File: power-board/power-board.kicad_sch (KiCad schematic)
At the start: 23 parts, among them J1 LINE/LOAD, J2 DISPLAY, J3 PROG, K1 G3MB-202P, Q1 2N2222A, U1 HLK-PM01, U2 Arduino_pro_mini, U3 MAX6675

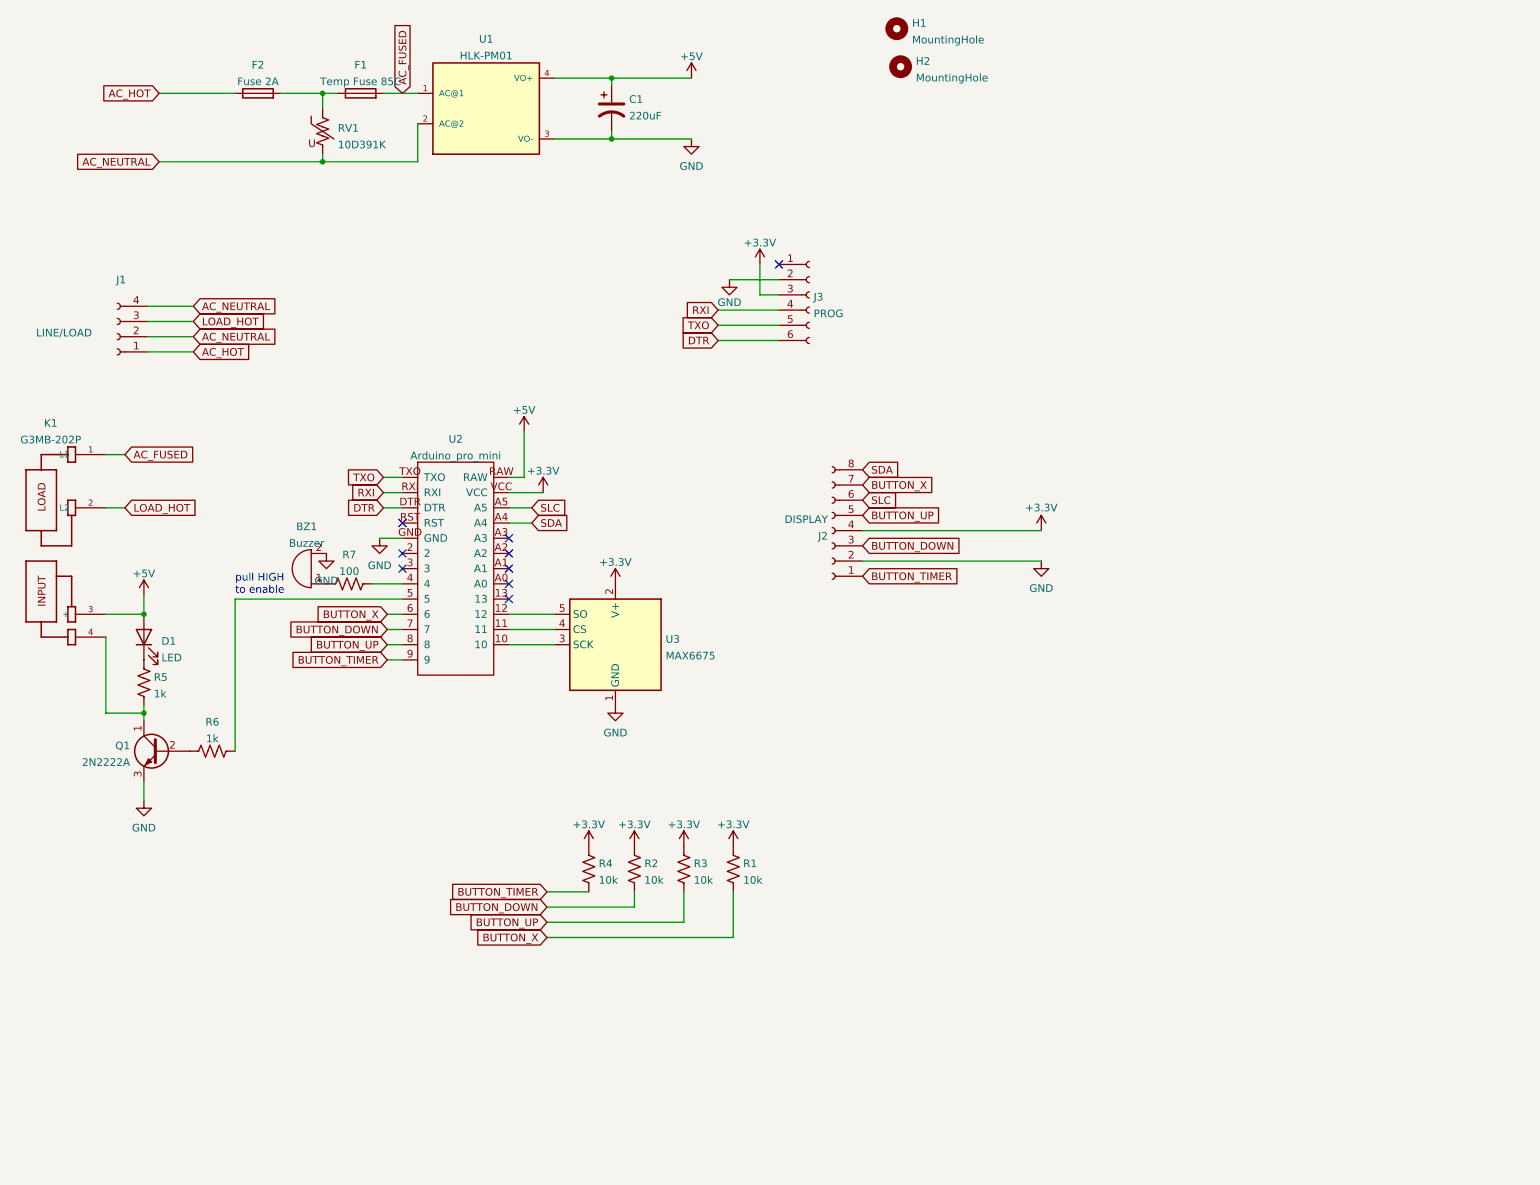
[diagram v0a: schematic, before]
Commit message: documentation
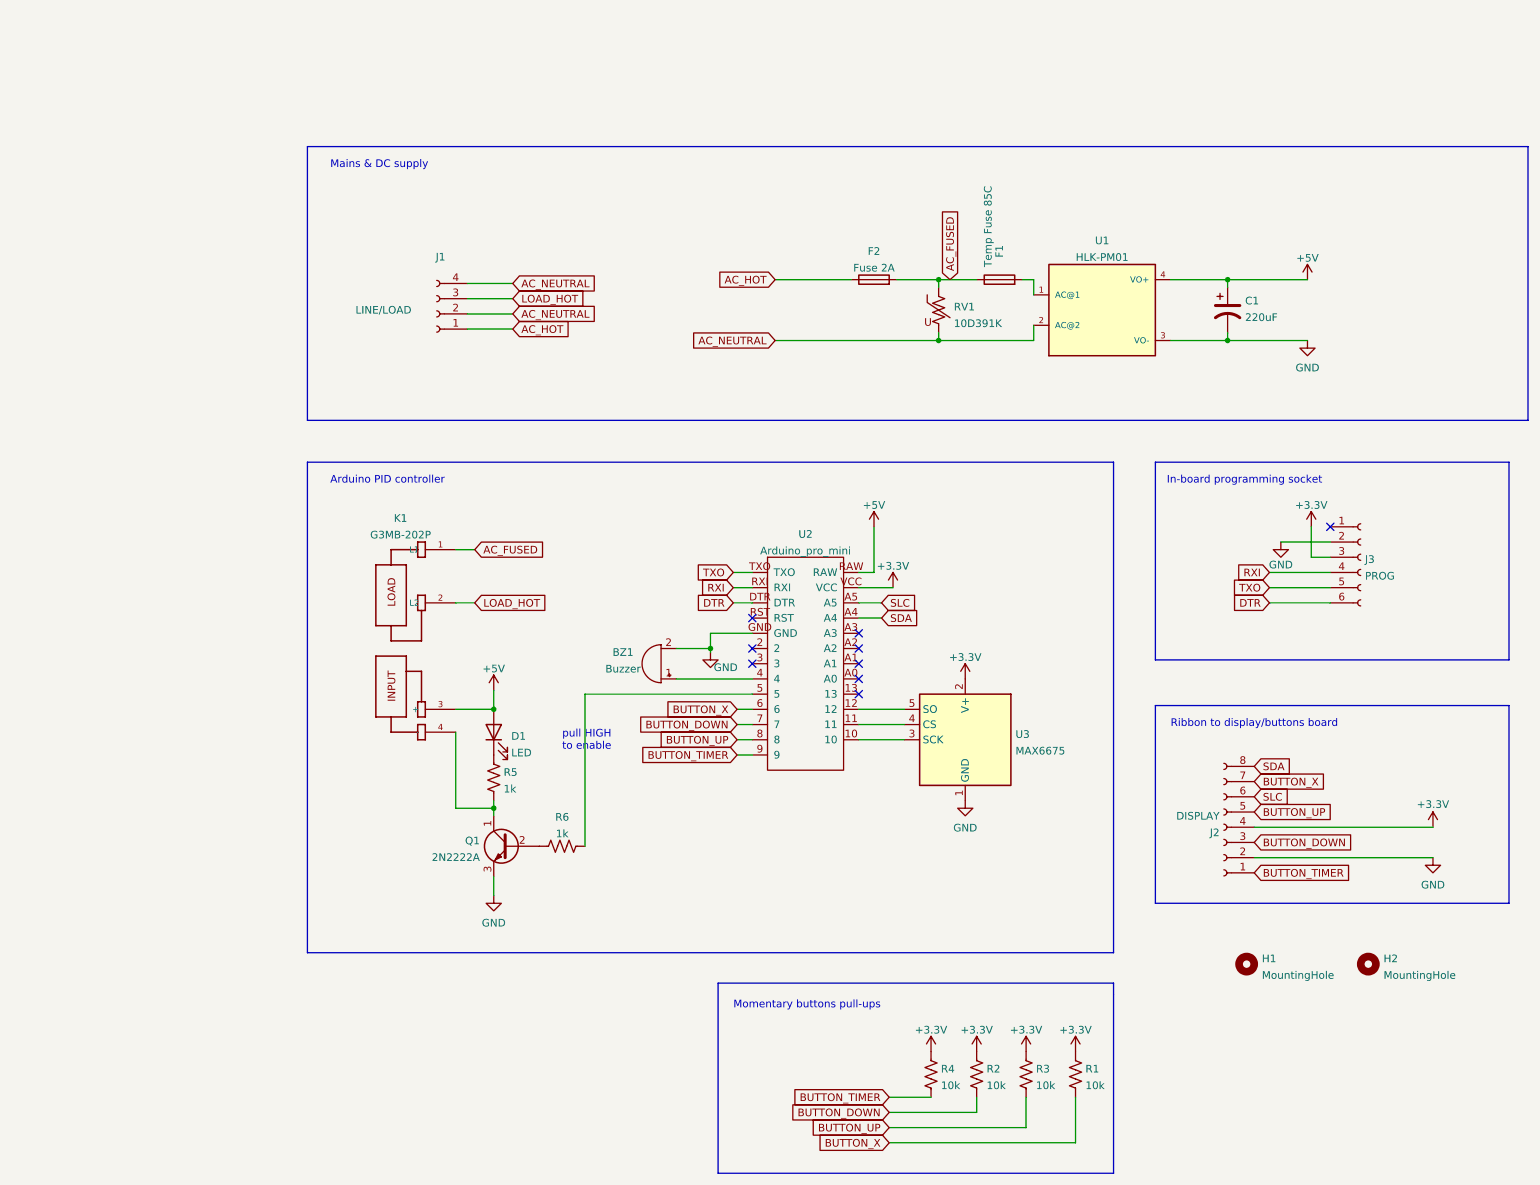
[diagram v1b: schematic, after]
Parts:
- removed R7: 100, Resistor_THT:R_Axial_DIN0204_L3.6mm_D1.6mm_P7.62mm_Horizontal, symbol Device:R_US
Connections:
- net AC_FUSED: now also F1.1, F2.2, RV1.1; no longer F1.2, U1.1 (AC@1)
- net at BZ1.1 (-): now also U2.4
- new net: F1.2, U1.1 (AC@1)
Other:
- note added: "Arduino PID controller"
- note added: "In-board programming socket"
- note added: "Mains & DC supply"
- note added: "Momentary buttons pull-ups"
- note added: "Ribbon to display/buttons board"
- moved on the sheet: BZ1, C1, D1, F1, F2, H1, H2, J1, J2, J3, K1, Q1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
